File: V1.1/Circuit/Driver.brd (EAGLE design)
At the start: 61.6 x 54.6 mm, 32 parts, among them IC1 DRV8300DIPWR, IC2 CD74HC4049PWR, U1 INA240A1PWR, U2 INA240A1PWR, U3 INA240A1PWR

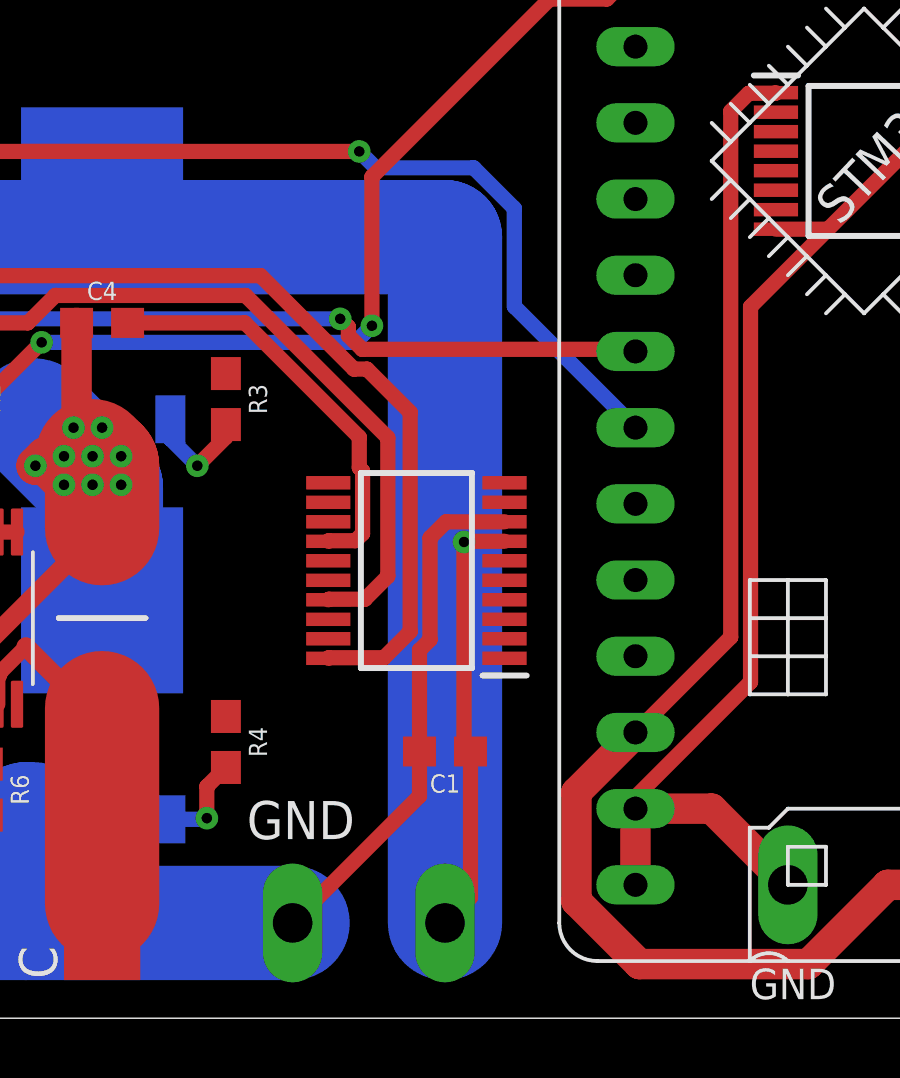
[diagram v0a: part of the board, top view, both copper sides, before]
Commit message: Ready for autoroutering 4
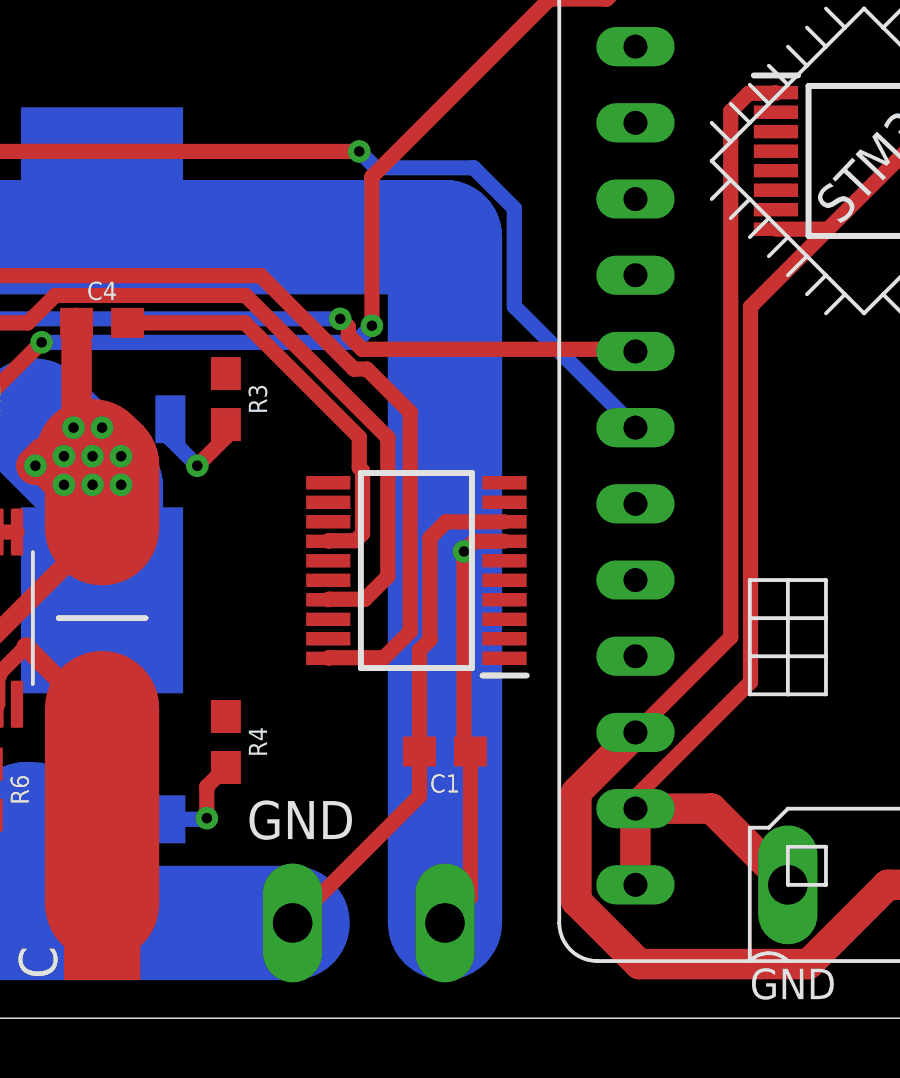
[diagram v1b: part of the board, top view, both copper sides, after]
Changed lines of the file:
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@@
 <wire x1="133.77" y1="11.6293125" x2="133.77" y2="8.255" width="0.508" layer="1"/>
 <wire x1="134.6575" y1="15.9125" x2="134.1213" y2="15.3763" width="0.508" layer="1"/>
-<wire x1="151.528" y1="28.915" x2="156.21" y2="49.53" width="0" layer="19" extent="1-1"/>
-<wire x1="133.77" y1="8.255" x2="140.97" y2="6.35" width="0" layer="19" extent="1-1"/>
-<wire x1="120.355" y1="9.83" x2="120.91" y2="5.995" width="0" layer="19" extent="1-16"/>
-<wire x1="111.465" y1="9.83" x2="112.02" y2="5.995" width="0" layer="19" extent="1-16"/>
-<wire x1="102.575" y1="9.83" x2="103.13" y2="5.995" width="0" layer="19" extent="1-16"/>
-<wire x1="119.055" y1="15.57" x2="120.355" y2="9.83" width="0" layer="19" extent="1-1"/>
-<wire x1="110.165" y1="15.57" x2="111.465" y2="9.83" width="0" layer="19" extent="1-1"/>
-<wire x1="101.275" y1="15.57" x2="102.575" y2="9.83" width="0" layer="19" extent="1-1"/>
 </signal>
 <signal name="3V3">
@@
 <wire x1="146.73386875" y1="1.1684" x2="141.09875625" y2="1.1684" width="1.016" layer="1"/>
 <wire x1="141.09875625" y1="1.1684" x2="139.0016" y2="3.26555625" width="1.016" layer="1"/>
-<wire x1="145.652" y1="30.215" x2="156.21" y2="52.07" width="0" layer="19" extent="1-1"/>
-<wire x1="120.355" y1="15.57" x2="140.97" y2="8.89" width="0" layer="19" extent="1-1"/>
-<wire x1="111.465" y1="15.57" x2="119.705" y2="15.57" width="0" layer="19" extent="1-1"/>
-<wire x1="102.575" y1="15.57" x2="110.815" y2="15.57" width="0" layer="19" extent="1-1"/>
 </signal>
 <signal name="RESET">
@@
 <contactref element="IC2" pad="3"/>
 <contactref element="U$1" pad="P$5"/>
-<wire x1="156.21" y1="13.97" x2="145.652" y2="28.915" width="0" layer="19" extent="1-1"/>
-<wire x1="136.6055" y1="11.3625" x2="145.652" y2="28.915" width="0" layer="19" extent="1-1"/>
 </signal>
 <signal name="INHB">
@@
 <contactref element="IC2" pad="5"/>
 <contactref element="U$1" pad="P$7"/>
-<wire x1="145.652" y1="27.615" x2="156.21" y2="19.05" width="0" layer="19" extent="1-1"/>
-<wire x1="136.6055" y1="12.0125" x2="145.652" y2="27.615" width="0" layer="19" extent="1-1"/>
 </signal>
 <signal name="INHC">
@@
 <contactref element="IC2" pad="7"/>
 <contactref element="U$1" pad="P$15"/>
-<wire x1="145.652" y1="26.315" x2="156.21" y2="39.37" width="0" layer="19" extent="1-1"/>
-<wire x1="136.6055" y1="12.6625" x2="145.652" y2="26.315" width="0" layer="19" extent="1-1"/>
 </signal>
 <signal name="INLA">
 <contactref element="IC1" pad="4"/>
 <contactref element="IC2" pad="2"/>
-<wire x1="136.6055" y1="13.3125" x2="145.652" y2="29.565" width="0" layer="19" extent="1-1"/>
 </signal>
 <signal name="INLB">
 <contactref element="IC1" pad="5"/>
 <contactref element="IC2" pad="4"/>
-<wire x1="136.6055" y1="13.9625" x2="145.652" y2="28.265" width="0" layer="19" extent="1-1"/>
 </signal>
 <signal name="INLC">
 <contactref element="IC1" pad="6"/>
 <contactref element="IC2" pad="6"/>
-<wire x1="136.6055" y1="14.6125" x2="145.652" y2="26.965" width="0" layer="19" extent="1-1"/>
 </signal>
 <signal name="GLC">
 <contactref element="IC1" pad="9"/>
 <contactref element="R4" pad="1"/>
-<wire x1="127.3175" y1="9.4225" x2="136.6055" y2="16.5625" width="0" layer="19" extent="1-1"/>
 </signal>
 <signal name="GLB">
 <contactref element="IC1" pad="10"/>
 <contactref element="R6" pad="1"/>
-<wire x1="119.38" y1="7.835" x2="136.6055" y2="17.2125" width="0" layer="19" extent="1-1"/>
 </signal>
 <signal name="BSTA">
@@
 <contactref element="IC1" pad="19"/>
 <contactref element="R1" pad="1"/>
-<wire x1="109.5375" y1="20.8525" x2="130.7295" y2="12.0125" width="0" layer="19" extent="1-1"/>
 </signal>
 <signal name="SHA">
@@
 <wire x1="104.56" y1="22.5425" x2="104.56" y2="18.63" width="1.016" layer="1"/>
 <wire x1="104.56" y1="18.63" x2="105.0925" y2="18.0975" width="1.016" layer="1"/>
-<wire x1="106.045" y1="17.145" x2="130.7295" y2="12.6625" width="0" layer="19" extent="1-1"/>
-<wire x1="105.0925" y1="17.145" x2="106.045" y2="17.145" width="0" layer="19" extent="1-1"/>
-<wire x1="104.14" y1="17.145" x2="105.0925" y2="17.145" width="0" layer="19" extent="1-1"/>
-<wire x1="105.0925" y1="18.0975" x2="106.045" y2="18.0975" width="0" layer="19" extent="1-1"/>
-<wire x1="101.275" y1="9.83" x2="101.2646" y2="9.83" width="0" layer="19" extent="1-1"/>
-<wire x1="103.13" y1="19.33" x2="104.4575" y2="19.05" width="0" layer="19" extent="16-16"/>
 </signal>
 <signal name="BSTB">
@@
 <contactref element="IC1" pad="16"/>
 <contactref element="R2" pad="1"/>
-<wire x1="118.4275" y1="20.8525" x2="130.7295" y2="13.9625" width="0" layer="19" extent="1-1"/>
 </signal>
 <signal name="SHB">
@@
 <wire x1="113.45" y1="22.5425" x2="113.45" y2="18.63" width="1.016" layer="1"/>
 <wire x1="113.45" y1="18.63" x2="113.9825" y2="18.0975" width="1.016" layer="1"/>
-<wire x1="114.935" y1="17.145" x2="130.7295" y2="14.6125" width="0" layer="19" extent="1-1"/>
-<wire x1="114.935" y1="18.0975" x2="114.935" y2="17.145" width="0" layer="19" extent="1-1"/>
-<wire x1="113.9825" y1="17.145" x2="114.935" y2="17.145" width="0" layer="19" extent="1-1"/>
-<wire x1="113.9825" y1="18.0975" x2="114.935" y2="18.0975" width="0" layer="19" extent="1-1"/>
-<wire x1="113.03" y1="18.0975" x2="113.03" y2="17.145" width="0" layer="19" extent="1-1"/>
-<wire x1="114.3" y1="19.05" x2="113.9825" y2="18.0975" width="0" layer="19" extent="1-1"/>
-<wire x1="113.3475" y1="19.05" x2="114.3" y2="19.05" width="0" layer="19" extent="1-1"/>
-<wire x1="112.02" y1="19.33" x2="113.3475" y2="19.05" width="0" layer="19" extent="16-16"/>
 </signal>
 <signal name="BSTC">
@@
 <contactref element="IC1" pad="13"/>
 <contactref element="R3" pad="1"/>
-<wire x1="130.7295" y1="15.9125" x2="127.3175" y2="20.8525" width="0" layer="19" extent="1-1"/>
 </signal>
 <signal name="SHC">
@@
 <wire x1="122.34" y1="22.5425" x2="122.34" y2="18.63" width="1.016" layer="1"/>
 <wire x1="122.34" y1="18.63" x2="122.8725" y2="18.0975" width="1.016" layer="1"/>
-<wire x1="123.825" y1="17.145" x2="130.7295" y2="16.5625" width="0" layer="19" extent="1-1"/>
-<wire x1="123.825" y1="18.0975" x2="123.825" y2="17.145" width="0" layer="19" extent="1-1"/>
-<wire x1="122.8725" y1="17.145" x2="123.825" y2="17.145" width="0" layer="19" extent="1-1"/>
-<wire x1="122.8725" y1="18.0975" x2="123.825" y2="18.0975" width="0" layer="19" extent="1-1"/>
-<wire x1="121.92" y1="18.0975" x2="121.92" y2="17.145" width="0" layer="19" extent="1-1"/>
-<wire x1="122.2375" y1="19.05" x2="121.92" y2="18.0975" width="0" layer="19" extent="1-1"/>
-<wire x1="123.19" y1="19.05" x2="122.2375" y2="19.05" width="0" layer="19" extent="1-1"/>
-<wire x1="120.91" y1="19.33" x2="122.2375" y2="19.05" width="0" layer="19" extent="16-16"/>
 </signal>
 <signal name="GLA">
 <contactref element="IC1" pad="11"/>
 <contactref element="R5" pad="1"/>
-<wire x1="130.7295" y1="17.2125" x2="110.49" y2="7.835" width="0" layer="19" extent="1-1"/>
 </signal>
 <signal name="VCC">
@@
 <contactref element="U$4" pad="3"/>
 <contactref element="VCC" pad="TP"/>
-<wire x1="134.62" y1="2.54" x2="134.62" y2="15.875" width="3.81" layer="16"/>
-<wire x1="134.62" y1="15.875" x2="134.62" y2="25.4" width="3.81" layer="16"/>
+<wire x1="134.62" y1="2.54" x2="134.62" y2="15.5575" width="3.81" layer="16"/>
+<wire x1="134.62" y1="15.5575" x2="134.62" y2="25.4" width="3.81" layer="16"/>
 <wire x1="134.62" y1="25.4" x2="105.41" y2="25.4" width="3.81" layer="16"/>
 <wire x1="105.41" y1="25.4" x2="105.41" y2="26.63" width="3.81" layer="16"/>
-<wire x1="136.6055" y1="15.2625" x2="135.2775" y2="15.2625" width="0.508" layer="1"/>
-<wire x1="135.2775" y1="15.2625" x2="135.255" y2="15.24" width="0.508" layer="1"/>
-<via x="135.255" y="15.24" extent="1-16" drill="0.35"/>
-<wire x1="135.255" y1="15.24" x2="134.62" y2="15.875" width="0.508" layer="16"/>
+<wire x1="136.6055" y1="15.2625" x2="135.595" y2="15.2625" width="0.508" layer="1"/>
+<wire x1="135.595" y1="15.2625" x2="135.255" y2="14.9225" width="0.508" layer="1"/>
+<via x="135.255" y="14.9225" extent="1-16" drill="0.35"/>
+<wire x1="135.255" y1="14.9225" x2="134.62" y2="15.5575" width="0.508" layer="16"/>
 <wire x1="135.47" y1="8.255" x2="135.47" y2="3.39" width="0.508" layer="1"/>
 <wire x1="135.47" y1="3.39" x2="134.62" y2="2.54" width="0.508" layer="1"/>
-<wire x1="135.255" y1="15.24" x2="135.255" y2="8.47" width="0.508" layer="1"/>
+<wire x1="135.255" y1="14.9225" x2="135.255" y2="8.47" width="0.508" layer="1"/>
 <wire x1="135.255" y1="8.47" x2="135.47" y2="8.255" width="0.508" layer="1"/>
-<wire x1="114.3" y1="26.63" x2="123.19" y2="26.63" width="0" layer="19" extent="16-16"/>
-<wire x1="105.41" y1="26.63" x2="114.3" y2="26.63" width="0" layer="19" extent="16-16"/>
 </signal>
 <signal name="N$1">
@@
 <contactref element="B" pad="1"/>
 <wire x1="114.3" y1="9.7" x2="114.3" y2="3.175" width="3.81" layer="1"/>
-<wire x1="110.8254" y1="9.83" x2="110.815" y2="9.83" width="0" layer="19" extent="1-1"/>
 </signal>
 <signal name="SLC">
@@
 <contactref element="C" pad="1"/>
 <wire x1="123.19" y1="9.7" x2="123.19" y2="3.175" width="3.81" layer="1"/>
-<wire x1="119.7154" y1="9.83" x2="119.705" y2="9.83" width="0" layer="19" extent="1-1"/>
 </signal>
 <signal name="SLA">
